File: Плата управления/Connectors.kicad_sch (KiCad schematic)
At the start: 14 parts, among them J1 A, J11 Conn_01x02_Pin, J12 Conn_01x02_Pin, J13 Conn_01x02_Pin, J14 Conn_01x02_Pin, J15 Conn_01x02_Pin, J2 B, J3 C, J4 Conn_01x02_Pin, J5 Conn_01x03_Pin, J6 Conn_02x04_Odd_Even, J7 Conn_01x02_Pin, J8 Conn_01x02_Pin, J9 Conn_01x02_Pin

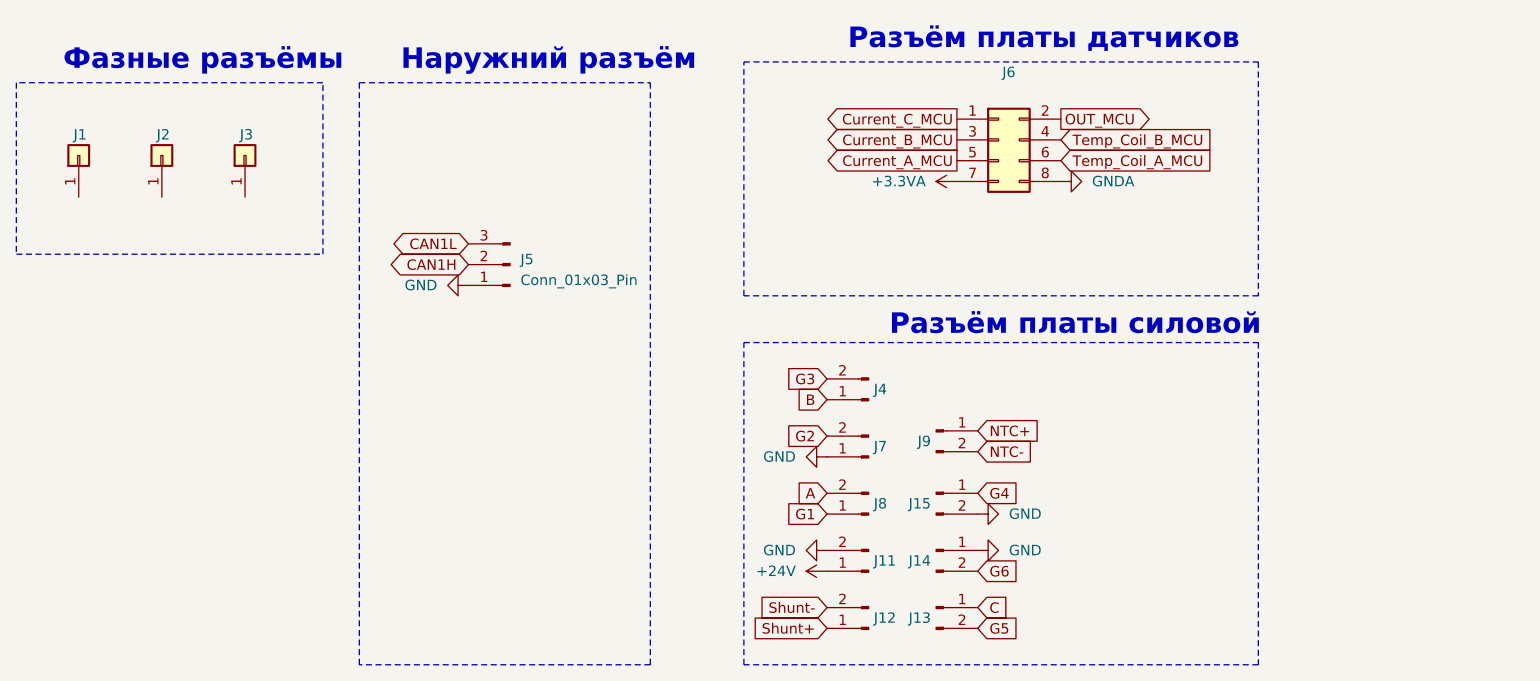
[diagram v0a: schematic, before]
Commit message: Новые драйвера и разъёмы
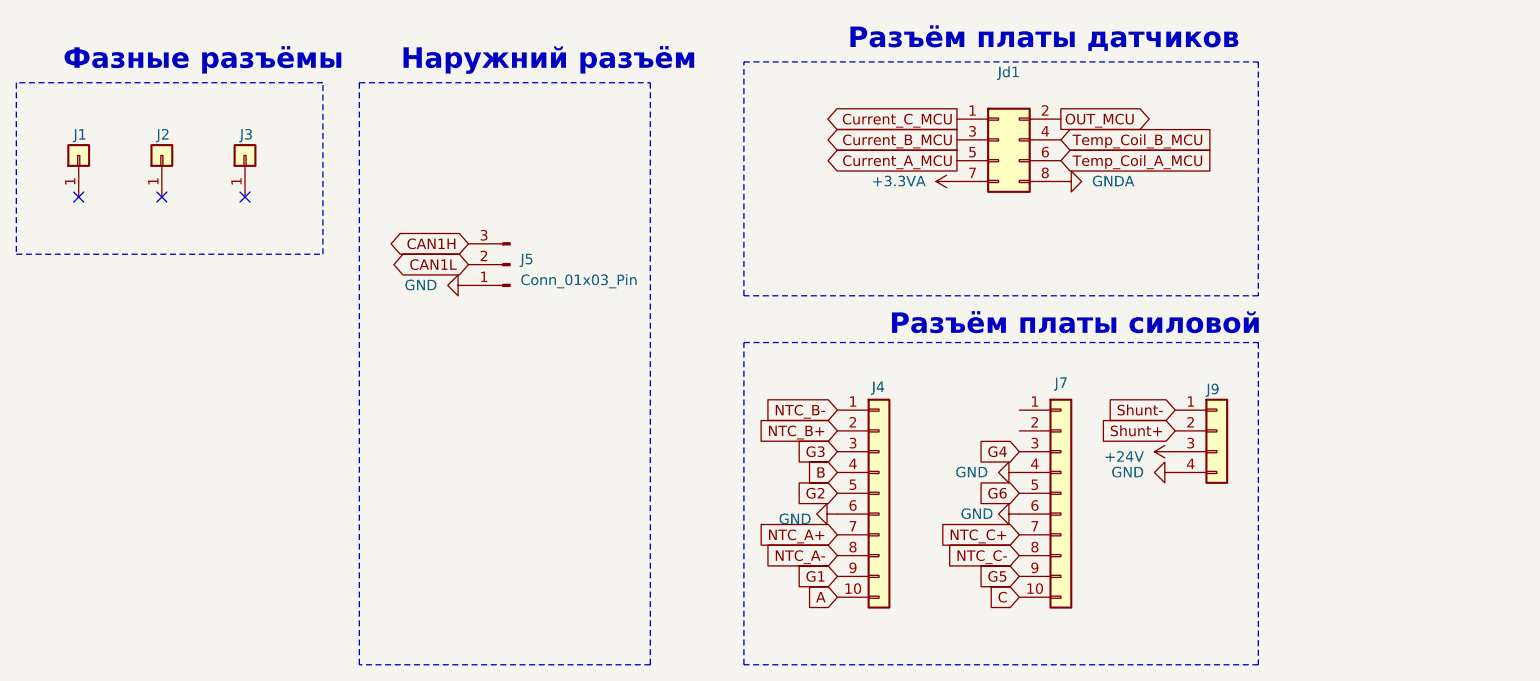
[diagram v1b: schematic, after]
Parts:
- removed J11, J12, J13, J14, J15, J4, J7, J8, J9: Conn_01x02_Pin, Connector_PinHeader_2.54mm:PinHeader_1x02_P2.54mm_Vertical, symbol Connector:Conn_01x02_Pin
- added J4, J7: Conn_01x10, Connector_PinHeader_1.27mm:PinHeader_1x10_P1.27mm_Vertical, symbol Connector_Generic:Conn_01x10
- added J9: Conn_01x04, Connector_PinHeader_1.27mm:PinHeader_1x04_P1.27mm_Vertical, symbol Connector_Generic:Conn_01x04
- J1, J2, J3: footprint Connector_My:Power_Wire -> Connector_My:Hole_9mm
- Jd1: renamed from J6; footprint Connector_PinHeader_2.00mm:PinHeader_2x04_P2.00mm_Vertical -> Connector_PinHeader_1.27mm:PinHeader_2x04_P1.27mm_Vertical
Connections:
- net +24V: now also J9.3 (Pin_3)
- net A: now also J4.10 (Pin_10)
- net B: now also J4.4 (Pin_4)
- net C: now also J7.10 (Pin_10)
- net CAN1H: now also J5.3 (Pin_3); no longer J5.2 (Pin_2)
- net CAN1L: now also J5.2 (Pin_2); no longer J5.3 (Pin_3)
- net G1: now also J4.9 (Pin_9)
- net G2: now also J4.5 (Pin_5)
- net G3: now also J4.3 (Pin_3)
- net G4: now also J7.3 (Pin_3)
- net G5: now also J7.9 (Pin_9)
- net G6: now also J7.5 (Pin_5)
- net GND: now also J4.6 (Pin_6), J7.4 (Pin_4), J7.6 (Pin_6), J9.4 (Pin_4)
- net Shunt+: now also J9.2 (Pin_2)
- net Shunt-: now also J9.1 (Pin_1)
- new net NTC_A+: J4.7 (Pin_7)
- new net NTC_A-: J4.8 (Pin_8)
- new net NTC_B+: J4.2 (Pin_2)
- new net NTC_B-: J4.1 (Pin_1)
- new net NTC_C+: J7.7 (Pin_7)
- new net NTC_C-: J7.8 (Pin_8)
- no-connect marks 0 -> 3
